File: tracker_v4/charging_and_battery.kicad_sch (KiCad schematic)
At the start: 20 parts, among them J1 USB_C_Receptacle_PowerOnly_6P, Q1 DMG9926UDM-7, U3 DW01A, U5 TP4056-42-ESOP8

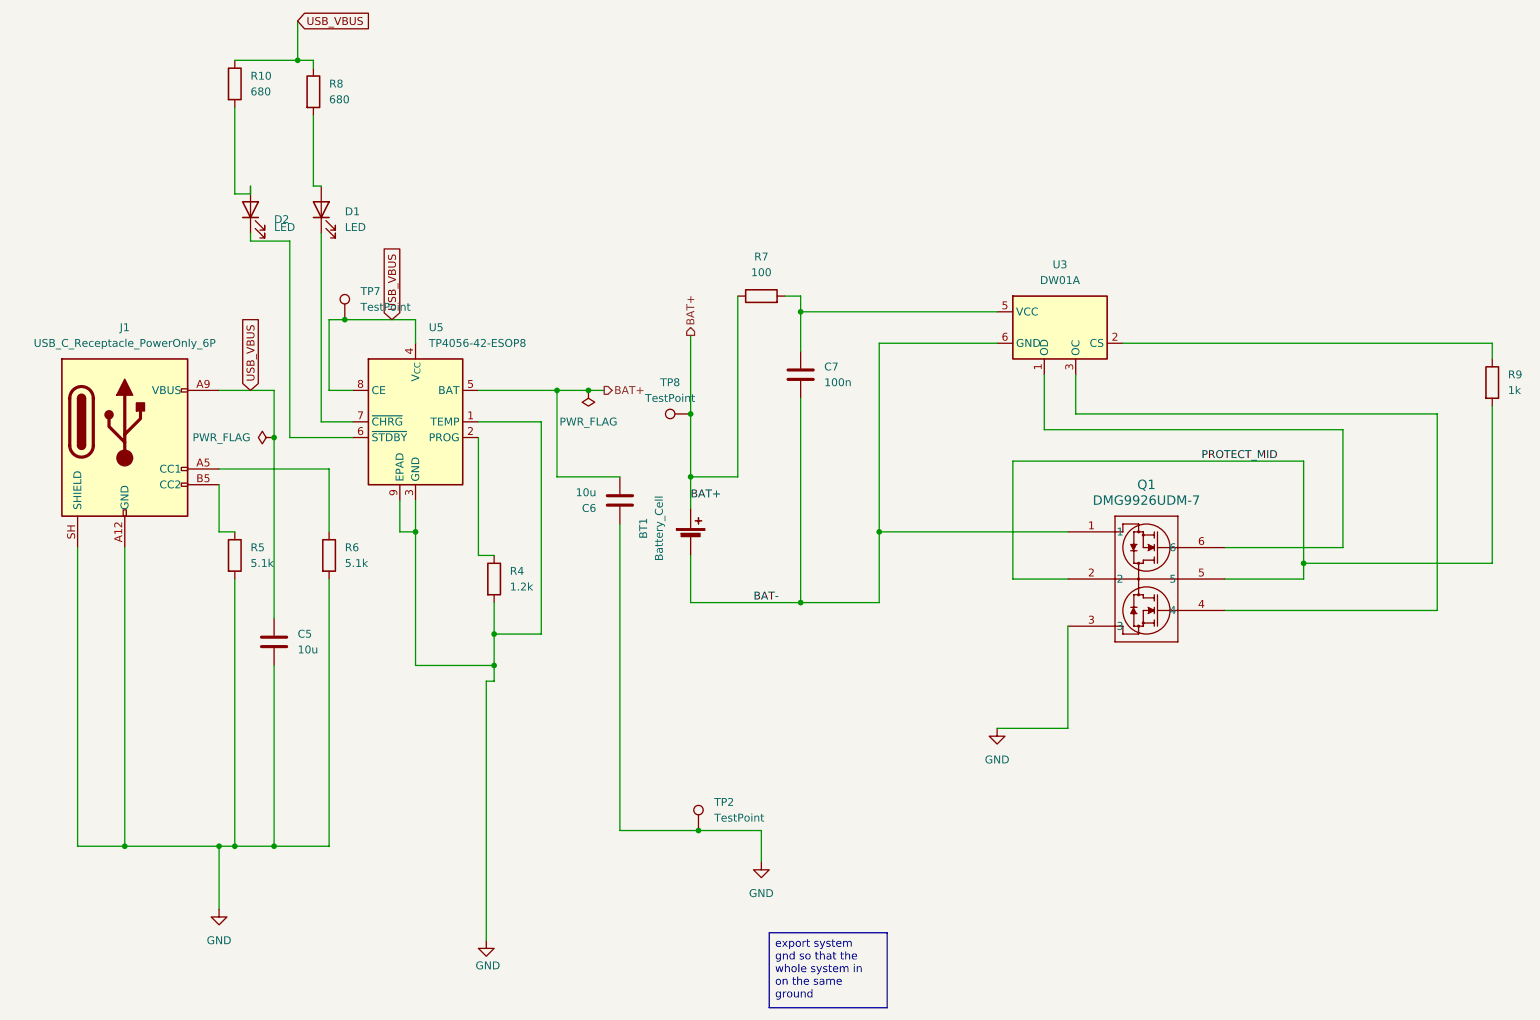
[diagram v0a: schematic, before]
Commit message: starting v4
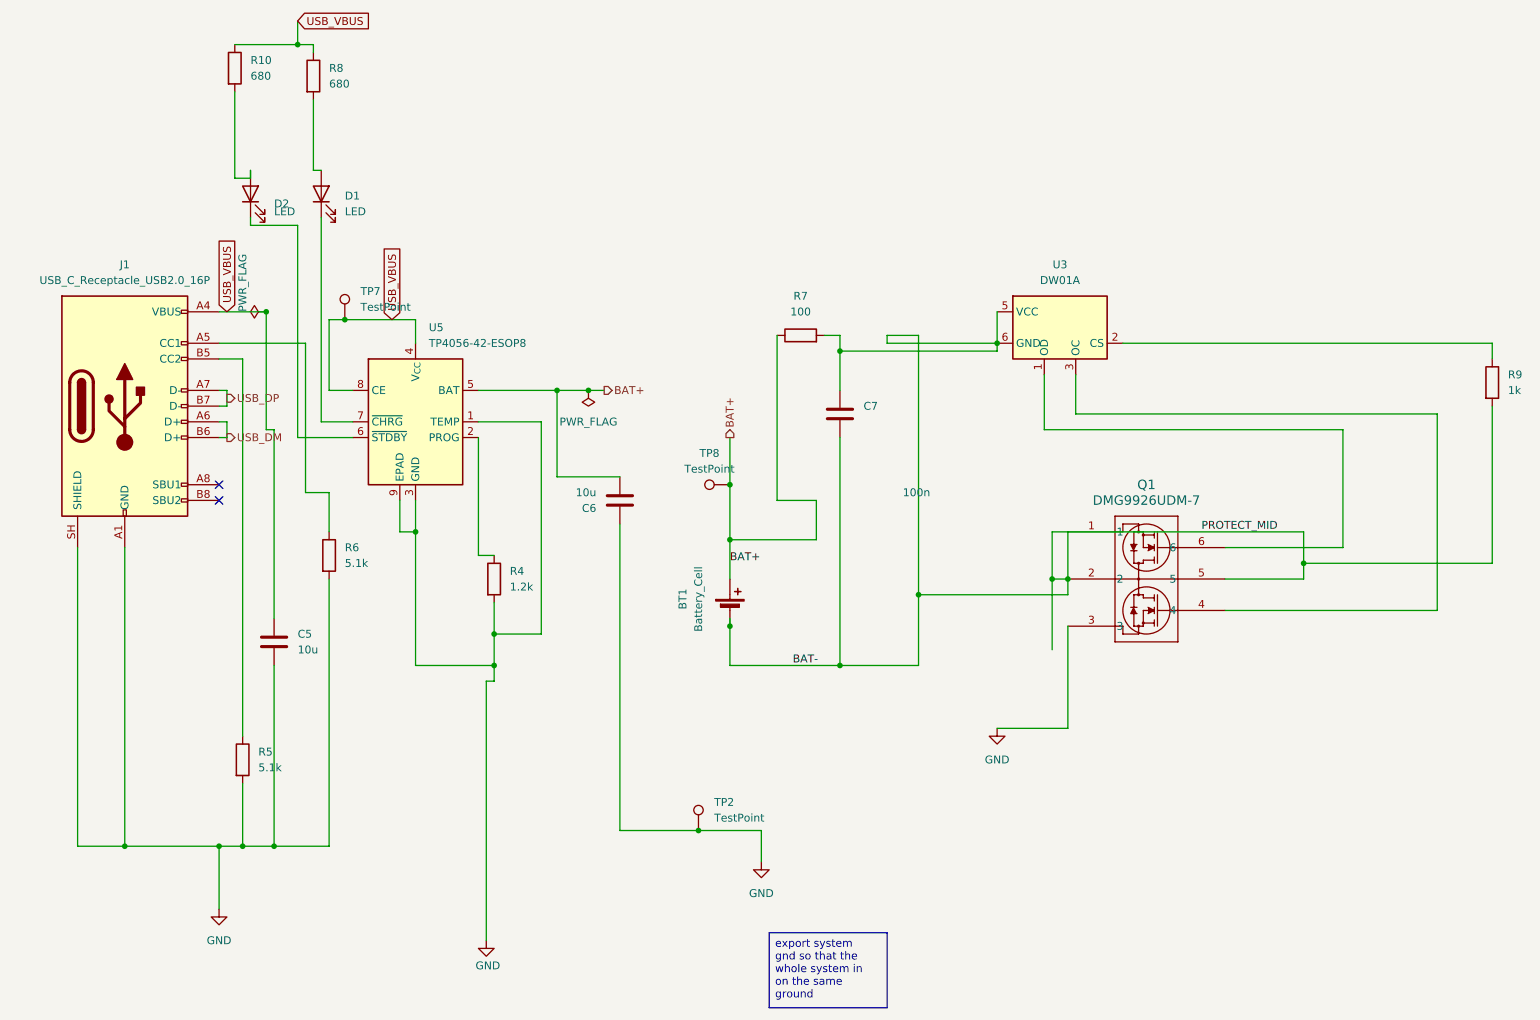
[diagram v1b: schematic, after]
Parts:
- removed J1: USB_C_Receptacle_PowerOnly_6P, Connector_USB:USB_C_Receptacle_GCT_USB4125-xx-x-0190_6P_TopMnt_Horizontal, symbol Connector:USB_C_Receptacle_PowerOnly_6P
- added J1: USB_C_Receptacle_USB2.0_16P, symbol Connector:USB_C_Receptacle_USB2.0_16P
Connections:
- net PROTECT_MID is gone; now on net BAT-: Q1.2, Q1.5, R9.2
- net BAT-: now also C7.1, R7.2, U3.5 (VCC)
- net GND: now also J1.A1 (GND), J1.A12 (GND), J1.B1 (GND), J1.B12 (GND), J1.SH (SHIELD)
- net USB_VBUS: now also J1.A4 (VBUS), J1.A9 (VBUS), J1.B4 (VBUS), J1.B9 (VBUS)
- net at R5.1: now also J1.B5 (CC2)
- net at R6.1: now also J1.A5 (CC1)
- new net USB_DM: J1.A6 (D+), J1.B6 (D+)
- new net USB_DP: J1.A7 (D-), J1.B7 (D-)
- no-connect marks 0 -> 2
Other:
- moved on the sheet: BT1, C7, D1, D2, R10, R5, R7, R8, TP8
